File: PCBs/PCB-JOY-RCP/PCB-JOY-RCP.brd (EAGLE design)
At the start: 21.8 x 55.5 mm, 27 parts, among them IC1 ADS7828, U2 MIC5205-3.3YM5

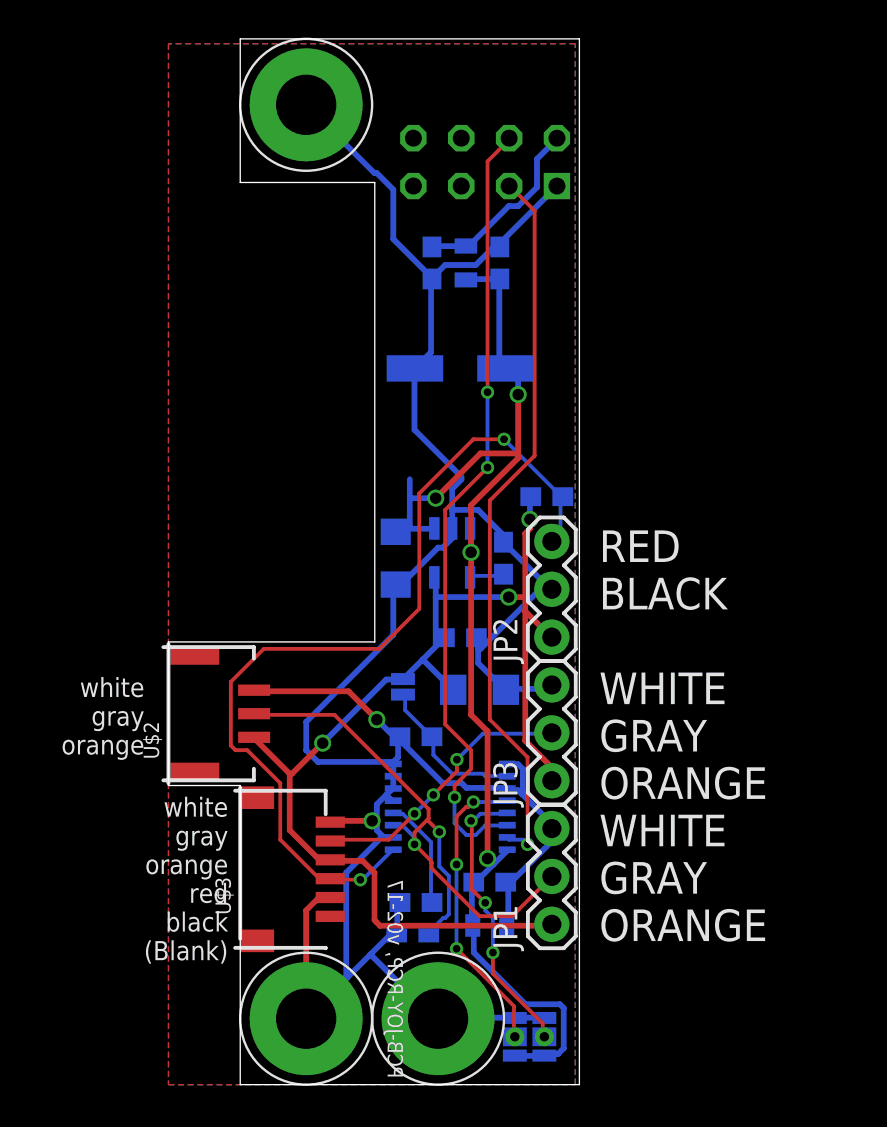
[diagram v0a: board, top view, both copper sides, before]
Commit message: update
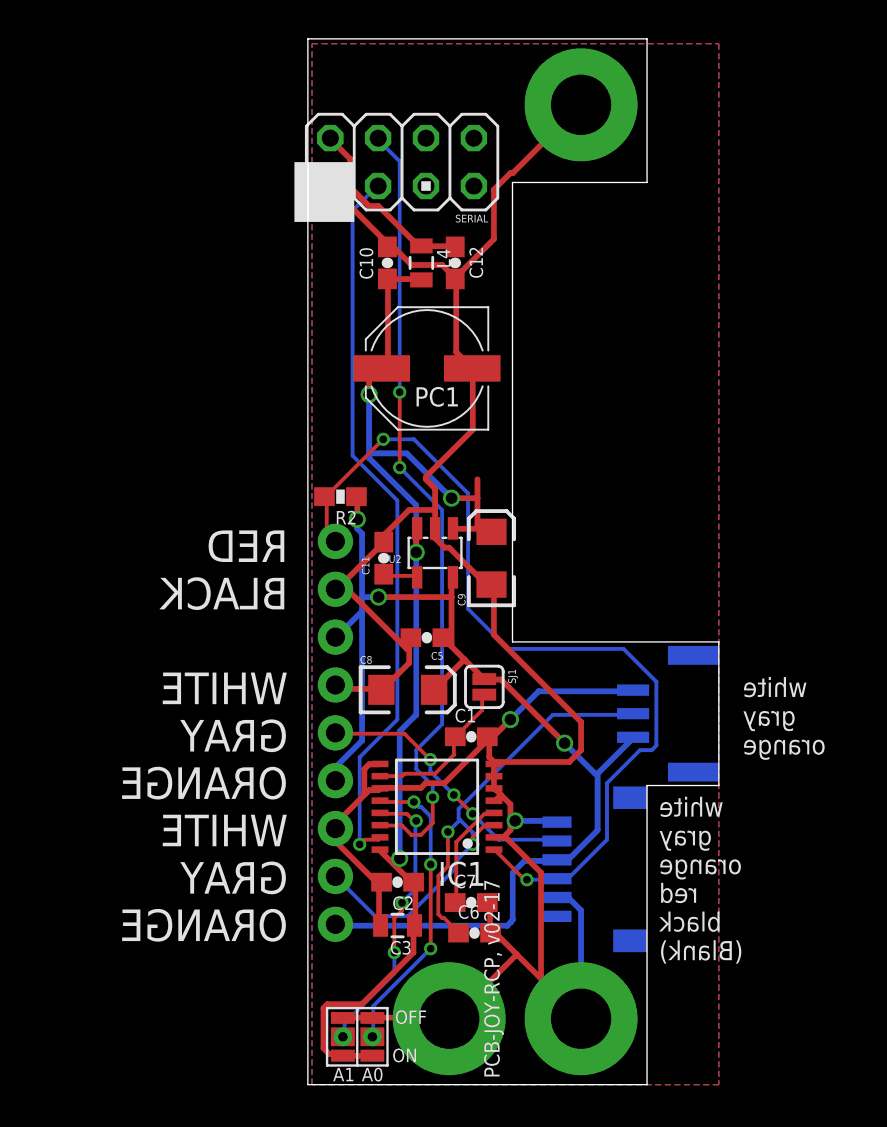
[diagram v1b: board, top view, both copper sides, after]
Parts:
- moved U$2 29.2 mm to (25.4, 19.7), flipped to the bottom
- moved U$3 21.6 mm to (21.6, 11.4), flipped to the bottom
- moved U$1 14.6 mm to (18.1, 3.50), flipped to the bottom
- moved U$6 14.6 mm to (18.1, 52.0), flipped to the bottom
- moved JP1 11.5 mm to (5.05, 8.51), flipped to the bottom
- moved JP2 11.5 mm to (5.05, 23.8), flipped to the bottom
- moved JP3 11.5 mm to (5.05, 16.1), flipped to the bottom
- moved R2 10.9 mm to (5.32, 31.2), flipped to the top
- moved U$19 10.7 mm to (5.45, 2.54), flipped to the top
- moved C11 6.35 mm to (7.62, 27.9), flipped to the top
- moved C10 5.96 mm to (7.82, 43.6), flipped to the top
- moved C9 5.08 mm to (13.3, 27.9), flipped to the top
- moved C2 4.89 mm to (8.35, 10.7), flipped to the top
- moved C3 4.89 mm to (8.35, 8.45), flipped to the top
- moved SERIAL 4.41 mm to (8.59, 49.0), flipped to the top
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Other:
- outline, holes or cut-outs redrawn
